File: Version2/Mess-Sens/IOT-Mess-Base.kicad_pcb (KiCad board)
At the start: 2 copper layers, 24.5 x 32.5 mm, 45 parts, among them IC1 SHT40I-AD1F-R2, J1 Conn_01x02_Pin, J2 TP_4056, J4 Conn_01x12_Pin, Q1 NM8205 PFETs, Q5 AO3401A, SW4 SW_Push, SW5 SW_Push, U1 TPL5110, U10 OPT3001DNPR, U11 HDC2010/DSBGA-6, U12 MMC5633NJL/WLP-4, U13 BH1750FVI-TR, U14 T117W, U15 DS1307Z+, U16 ENS210, U17 LIS2MDL, U19 MTS4, U2 INA219AxDCN, U3 TLV493D, U4 INA219AxD, U5 SHT31-DIS, U6 APDS-9960, U7 QMC6309/WLCSP-4, U8 AND_Gate, U9 LTR-303ALS-01

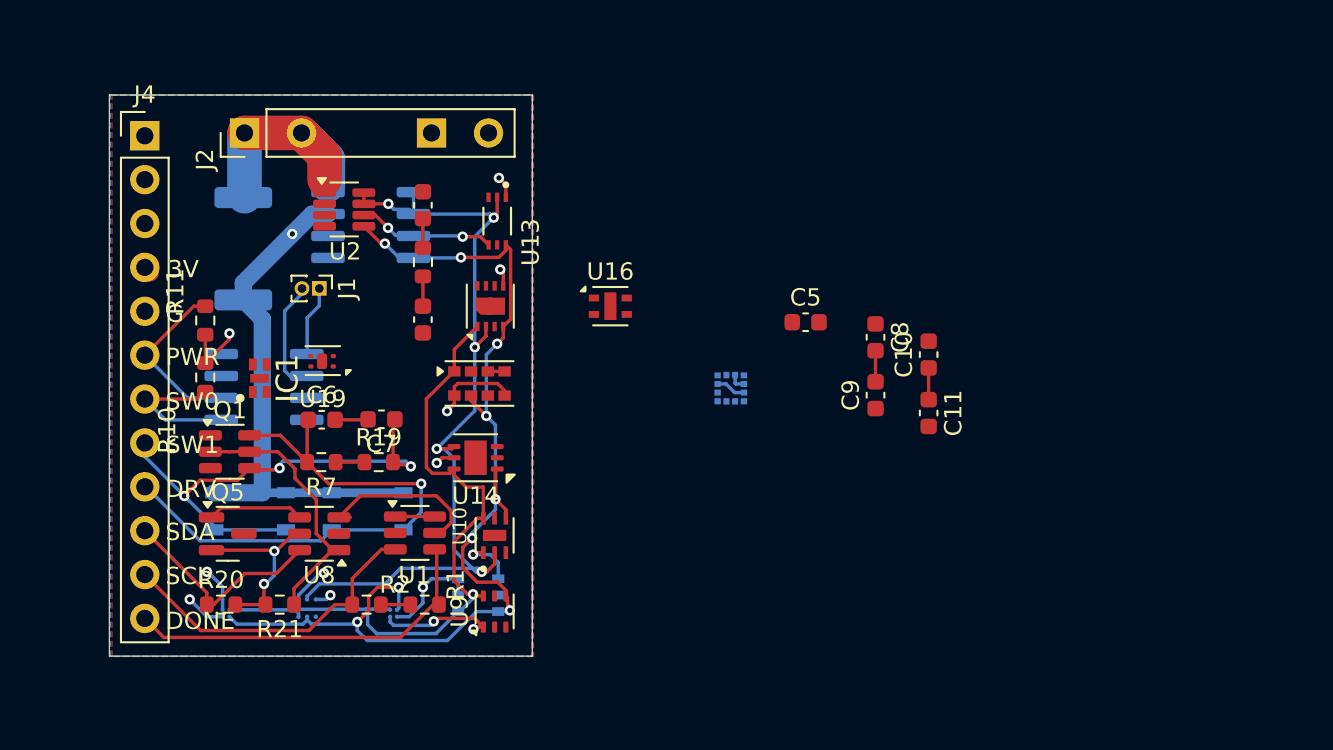
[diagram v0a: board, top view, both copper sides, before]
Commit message: updated.
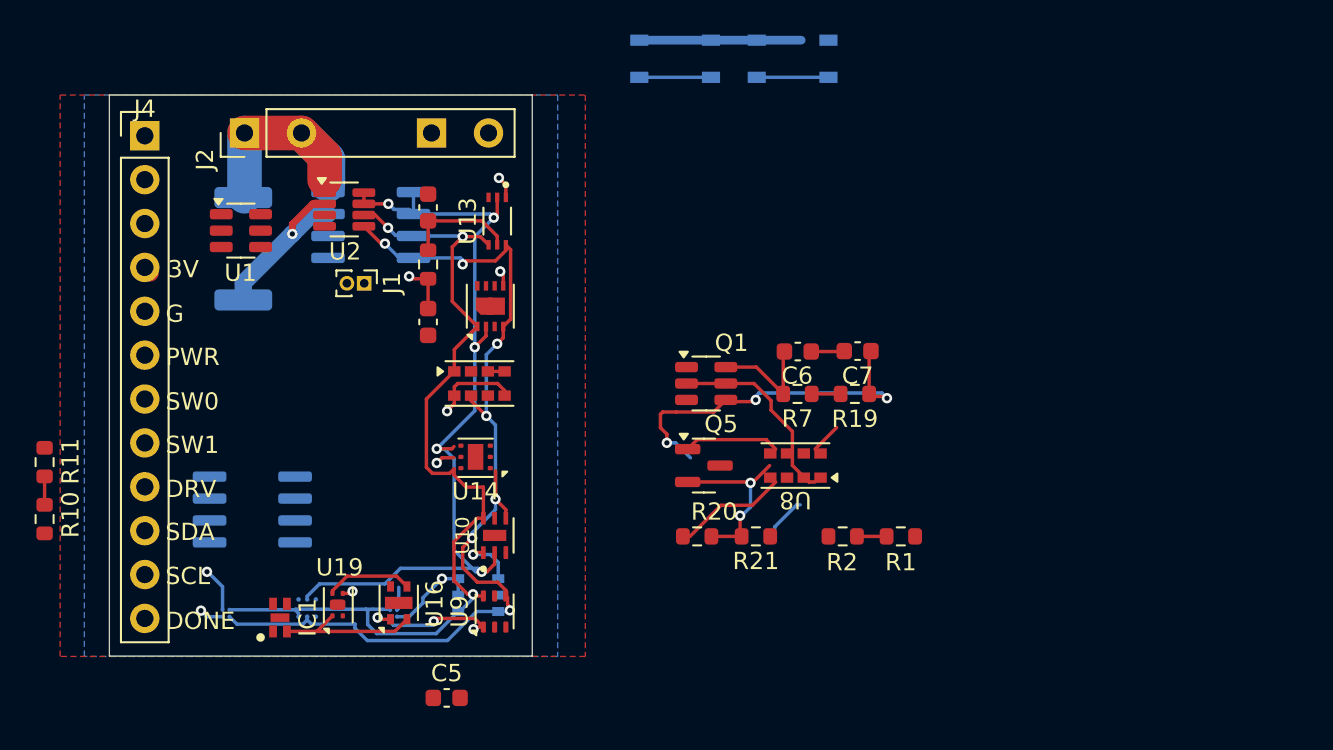
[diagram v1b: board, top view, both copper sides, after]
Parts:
- removed C10, C11: .1u, Capacitor_SMD:C_0603_1608Metric
- removed C8: .22u, Capacitor_SMD:C_0603_1608Metric
- removed C9: 10u, Capacitor_SMD:C_0603_1608Metric
- removed U17: LIS2MDL, Package_LGA:LGA-12_2x2mm_P0.5mm
- U14: footprint Package_DFN_QFN:TDFN-6-1EP_2.5x2.5mm_P0.65mm_EP1.3x2mm -> IOT-Mess-Footprints:DFN-6L
- U8: footprint Package_TO_SOT_SMD:SOT-23-6 -> Sensor:Avago_APDS-9960
- moved SW4 35.9 mm to (118.3, 60.5)
- moved SW5 35.9 mm to (111.5, 60.5)
- moved C5 30.1 mm to (98.3, 97.5)
- moved C7 27.8 mm to (122.1, 77.4)
- moved Q1 27.8 mm to (113.3, 79.3)
- moved Q5 27.8 mm to (113.2, 84.1)
- moved R19 27.8 mm to (121.9, 79.9)
- moved R2 27.8 mm to (121.2, 88.1)
- moved R20 27.8 mm to (112.8, 88.2)
- moved R21 27.8 mm to (116.2, 88.2)
- moved R7 27.8 mm to (118.6, 79.9)
- moved C6 27.8 mm to (118.6, 77.5)
- moved R1 27.8 mm to (124.6, 88.2)
- moved U8 27.8 mm to (118.5, 84.1)
- moved U16 21.1 mm to (95.5, 92.0), turned to 90 degrees
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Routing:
- net LSW0: track 33.4 -> 10.8 mm, vias 1 -> 0
- net DONE: track 21.6 -> 0.18 mm
- net R_DELAY: track 18.7 -> 0.00 mm
- net Vb: track 45.8 -> 30.2 mm
- net Net-(U1-DRV): track 10.3 -> 1.77 mm
- net Net-(J1-Pin_2): track 6.58 -> 0.00 mm
- net EN: track 12.7 -> 6.68 mm
- net SCL_0: track 72.2 -> 67.1 mm, vias 9 -> 7
- net GND: track 17.6 -> 12.6 mm, vias 3 -> 2
- net Net-(U13-DVI): track 1.70 -> 6.57 mm
- net Net-(U8-A): track 15.7 -> 11.3 mm
- net Net-(J1-Pin_1): track 4.10 -> 0.00 mm
- net +3.3V: track 32.7 -> 29.3 mm, vias 10 -> 11
- net LSW1: track 28.6 -> 25.3 mm
- net SDA_0: track 56.6 -> 59.1 mm

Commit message: did some works.
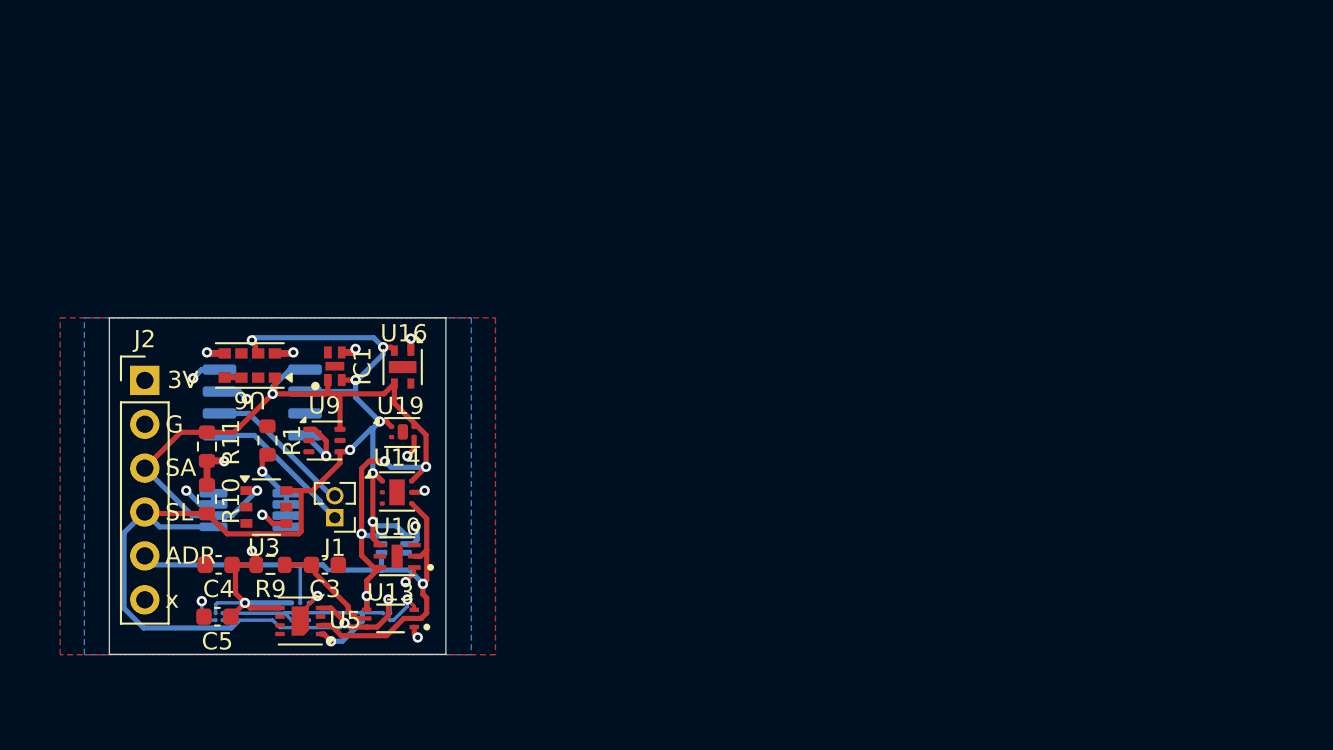
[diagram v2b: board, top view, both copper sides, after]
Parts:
- removed C6, C7: 0.1u, Capacitor_SMD:C_0603_1608Metric
- removed J4: Conn_01x12_Pin, Connector_PinHeader_2.54mm:PinHeader_1x12_P2.54mm_Vertical
- removed Q1: NM8205 PFETs, Package_TO_SOT_SMD:SOT-23-6
- removed Q5: AO3401A, Package_TO_SOT_SMD:SOT-23
- removed R19, R2, R20, R21, R7: R, Resistor_SMD:R_0603_1608Metric
- removed R4: 0.1R, Resistor_SMD:R_2512_6332Metric
- removed SW4, SW5: SW_Push, Button_Switch_SMD:SW_SPST_PTS810
- removed U2: INA219AxDCN, Package_TO_SOT_SMD:SOT-23-8
- removed U8: AND_Gate, Sensor:Avago_APDS-9960
- C3: value 0.1u -> 0.1uF
- C4: value 1u -> 1uF
- J1: footprint Connector_PinHeader_1.00mm:PinHeader_1x02_P1.00mm_Vertical -> Connector_PinHeader_1.27mm:PinHeader_1x02_P1.27mm_Vertical
- J2: value TP_4056 -> Conn_01x06_Pin; footprint IOT-Mess-Footprints:TP_Charger -> Connector_PinHeader_2.54mm:PinHeader_1x06_P2.54mm_Vertical
- R1: value R -> 10K
- U1: value TPL5110 -> TMP102xxDRL; footprint Package_TO_SOT_SMD:SOT-23-6 -> Package_TO_SOT_SMD:SOT-563; moved to B.Cu
- U3: moved to F.Cu
- U4: value INA219AxD -> TMP1075DGK; footprint Package_SO:SOIC-8_3.9x4.9mm_P1.27mm -> Package_SO:VSSOP-8_3x3mm_P0.65mm
- moved R1 37.1 mm to (87.9, 82.6), turned to -90 degrees
- moved U13 23.8 mm to (95.0, 92.9), turned to 180 degrees
- moved C3 21.5 mm to (91.2, 89.8), turned to 0 degrees
- moved U5 21.3 mm to (89.8, 93.0), turned to 180 degrees
- moved U1 20.2 mm to (95.2, 88.6), turned to 180 degrees
- moved R9 19.6 mm to (88.1, 89.8), turned to 0 degrees
- moved C4 18.6 mm to (85.1, 89.8), turned to 180 degrees
- moved U4 17.9 mm to (86.9, 86.6), turned to 0 degrees
- moved J2 15.4 mm to (80.8, 79.1), turned to 0 degrees
- moved IC1 14.9 mm to (91.8, 78.3)
- moved C5 14.1 mm to (85.0, 92.8), turned to 180 degrees
- moved U9 14.0 mm to (91.2, 82.6), turned to 0 degrees
- moved J1 13.7 mm to (91.8, 87.1), turned to 180 degrees
- moved U16 13.7 mm to (95.7, 78.3), turned to -90 degrees
- moved U6 13.3 mm to (86.9, 78.3), turned to 180 degrees
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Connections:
- J2 pad 1: Va -> +3.3V
- J2 pad 2: Va -> GND
- J2 pad 3: unconnected-(J2-Pin_3-Pad3) -> SDA_0
- J2 pad 4: GND -> SCL_0
- R1 pad 1: GND -> unconnected-(R1-Pad1)
- R1 pad 2: DONE -> Net-(U4-A0)
- R10 pad 1: SDA_0 -> SCL_0
- R11 pad 2: SCL_0 -> SDA_0
- U1 pad 1: Vb -> SCL_0
- U1 pad 3: R_DELAY -> unconnected-(U1-ALERT-Pad3)
- U1 pad 4: DONE -> ADDR
- U1 pad 5: Net-(U1-DRV) -> +3.3V
- U1 pad 6: Vb -> SDA_0
- U14 pad 7: (no net) -> GND
- U4 pad 1: ADDR -> SCL_0
- U4 pad 2: ADDR -> SDA_0
- U4 pad 3: SDA_0 -> GND
- U4 pad 4: SCL_0 -> GND
- U4 pad 5: +3.3V -> Net-(U4-A0)
- U4 pad 6: GND -> Net-(U4-A0)
- U4 pad 7: Vb -> Net-(U4-A0)
- U4 pad 8: Va -> +3.3V
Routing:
- net Vb: track 30.2 -> 0.00 mm, vias 3 -> 0
- net LSW1: track 25.3 -> 0.00 mm, vias 3 -> 0
- net ADDR: track 49.6 -> 34.7 mm, vias 5 -> 1
- net SCL_0: track 67.1 -> 81.2 mm, vias 7 -> 9
- net Va: track 13.9 -> 0.00 mm
- net Net-(U8-A): track 11.3 -> 0.00 mm
- net LSW0: track 10.8 -> 0.00 mm
- net Net-(J1-Pin_1): track 0.00 -> 8.71 mm
- net Net-(J1-Pin_2): track 0.00 -> 8.65 mm
- net SDA_0: track 59.1 -> 67.8 mm, vias 3 -> 7
- net EN: track 6.68 -> 0.00 mm
- net Net-(Q5-G): track 5.56 -> 0.00 mm
- net Net-(U4-A0): track 0.00 -> 4.32 mm, vias 0 -> 1
- net Net-(U1-DRV): track 1.77 -> 0.00 mm
- net +3.3V: track 29.3 -> 30.6 mm, vias 11 -> 14
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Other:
- board size 24.5 x 32.5 mm -> 19.5 x 19.5 mm
- board text added: "ADR"
- board text added: "IOT-Mess SENS V2.0 8/18/25"
- board text added: "SA"
- board text added: "SL"
- board text added: "x"
- board text removed: "DONE"
- board text removed: "DRV"
- board text removed: "IOT-Mess SENS V1.0 7/5/25"
- board text removed: "PWR"
- board text removed: "SCL"
- board text removed: "SDA"
- board text removed: "SW0"
- board text removed: "SW1"

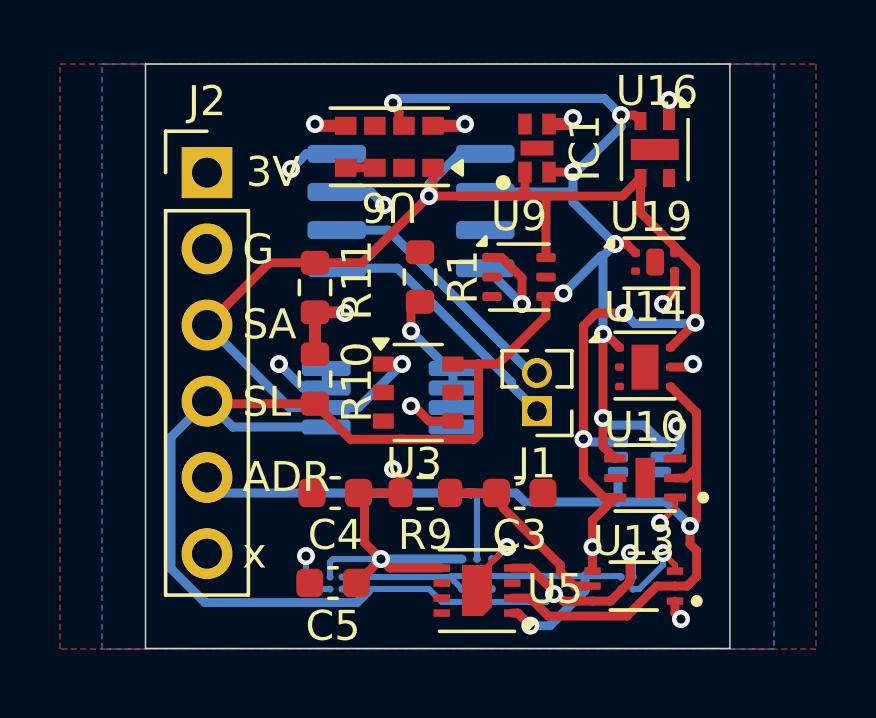
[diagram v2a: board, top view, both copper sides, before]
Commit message: update stuff.
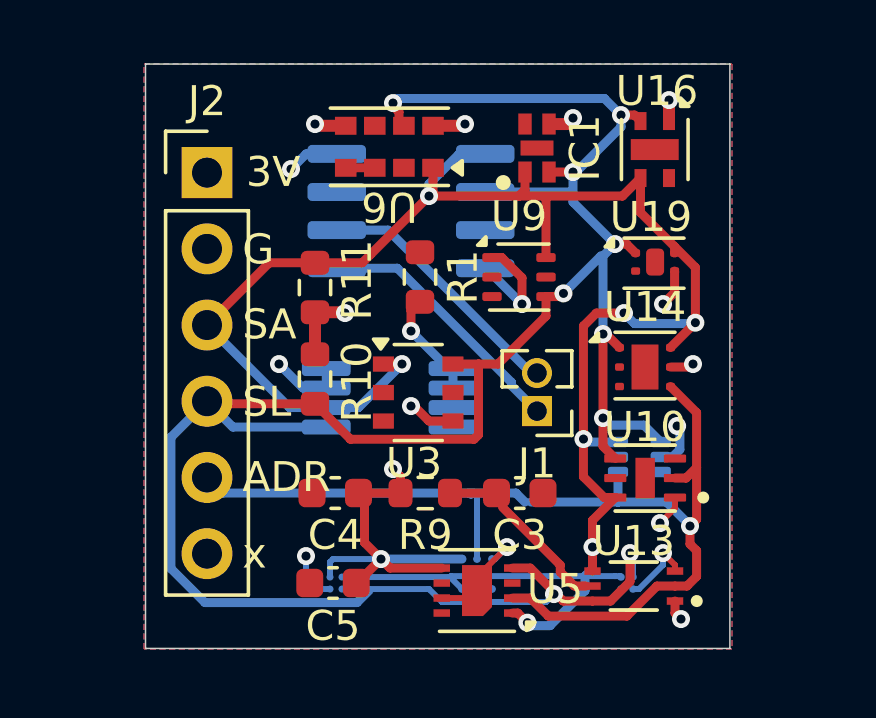
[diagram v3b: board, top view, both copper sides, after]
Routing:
- net +3.3V: track 30.6 -> 28.9 mm, vias 14 -> 13
- net GND: track 12.5 -> 13.8 mm

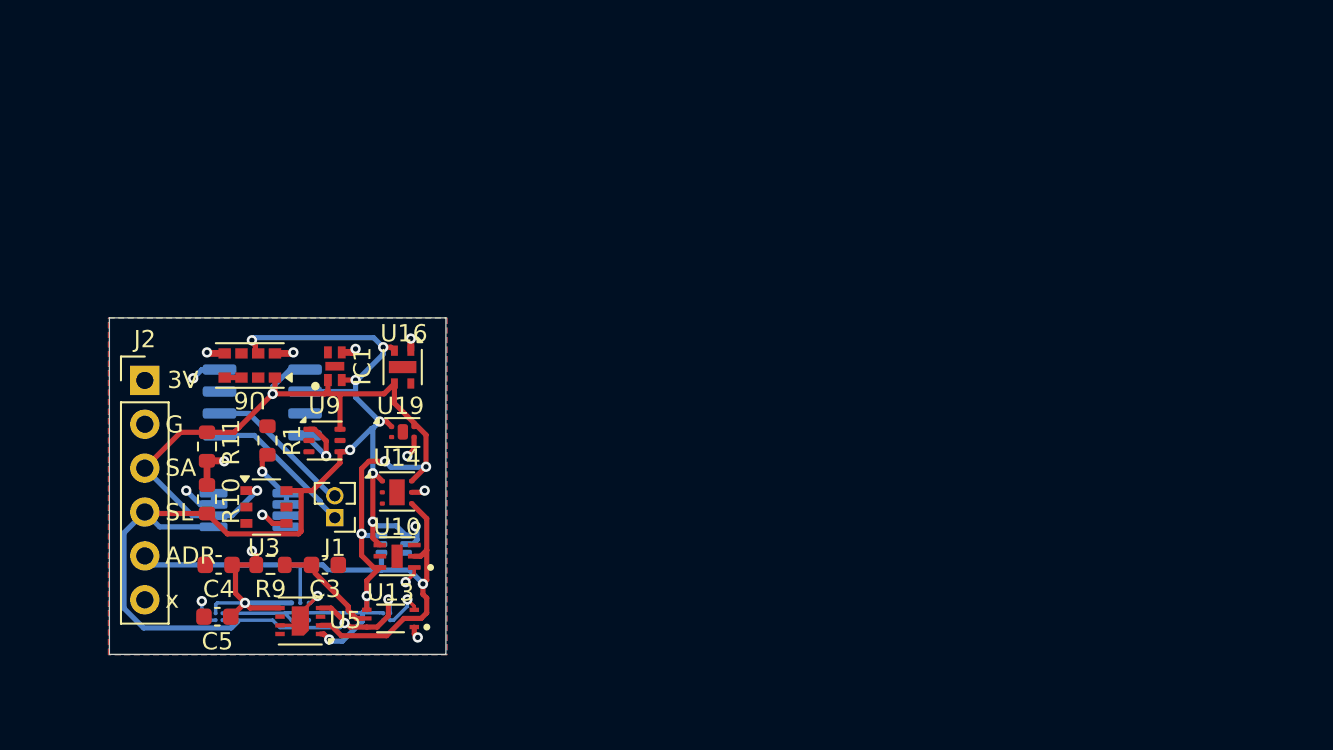
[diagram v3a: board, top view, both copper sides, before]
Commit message: updates.
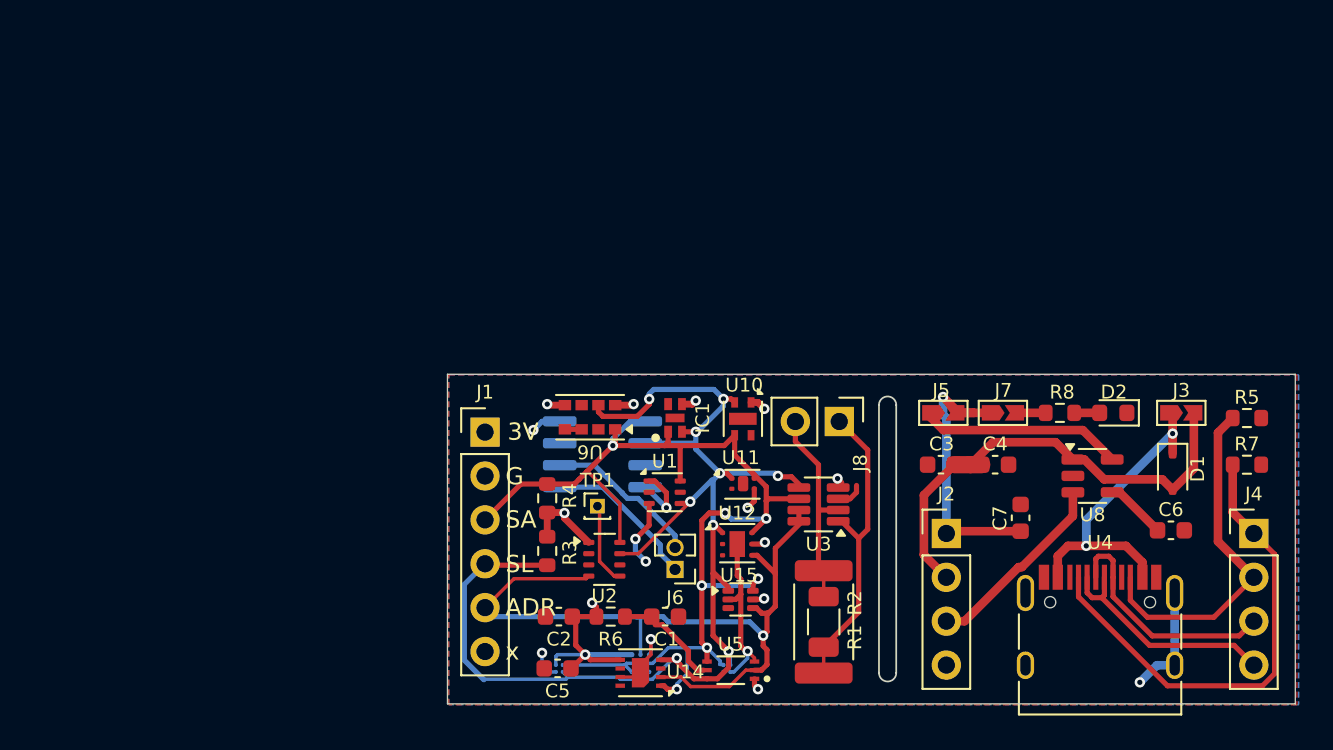
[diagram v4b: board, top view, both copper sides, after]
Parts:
- removed the U10 at (95.4, 89.3)
- added C3: 10u, Capacitor_SMD:C_0603_1608Metric, F.Cu at (126.9, 84.0)
- added C4: 1u, Capacitor_SMD:C_0603_1608Metric, F.Cu at (130.0, 84.0)
- added C6: 22nF, Capacitor_SMD:C_0603_1608Metric, F.Cu at (140.2, 87.8)
- added C7: 1u, Capacitor_SMD:C_0603_1608Metric, F.Cu at (131.5, 87.1)
- added D1: 1N5819WS, Diode_SMD:D_SOD-323, F.Cu at (140.3, 84.4)
- added D2: LED, LED_SMD:LED_0603_1608Metric, F.Cu at (136.9, 81.0)
- added J2: Conn_01x04_Pin, Connector_PinHeader_2.54mm:PinHeader_1x04_P2.54mm_Vertical, F.Cu at (127.2, 88.0)
- added J3: Jumper_2, IOT-Mess-Footprints:Jumpper-triangle, F.Cu at (140.8, 81.0)
- added J4: Conn_01x04_Pin, Connector_PinHeader_2.54mm:PinHeader_1x04_P2.54mm_Vertical, F.Cu at (145.0, 88.0)
- added J5: Jumper_2, IOT-Mess-Footprints:Jumpper-triangle, F.Cu at (127.0, 81.0)
- added J7: Jumper_2, IOT-Mess-Footprints:Jumpper-triangle, F.Cu at (130.5, 81.0)
- added J8: Conn_01x02_Pin, Connector_PinHeader_2.54mm:PinHeader_1x02_P2.54mm_Vertical, F.Cu at (121.0, 81.5)
- added R2: 0.1, Resistor_SMD:R_1206_3216Metric, F.Cu at (120.1, 93.1)
- added R5: 5.1K, Resistor_SMD:R_0603_1608Metric, F.Cu at (144.6, 81.3)
- added R7: 5.1K, Resistor_SMD:R_0603_1608Metric, F.Cu at (144.6, 84.0)
- added R8: R, Resistor_SMD:R_0603_1608Metric, F.Cu at (133.8, 81.0)
- added TP1: TestPoint, Connector_PinHeader_1.00mm:PinHeader_1x01_P1.00mm_Vertical, F.Cu at (107.0, 86.4)
- added U2: LTR-507ALS, IOT-Mess-Footprints:LTR-507ALS, F.Cu at (106.5, 88.5)
- added U8: ME6211C33M5, Package_TO_SOT_SMD:SOT-23-5, F.Cu at (135.7, 84.7)
- R1: value 10K -> 0.1; footprint Resistor_SMD:R_0603_1608Metric -> Resistor_SMD:R_2512_6332Metric
- U1: renamed from U9; value LTR-303ALS-01 -> LTR-303/308
- U11: renamed from U19; value MTS4 -> MTS4 0.1C DFN-4L
- U12: renamed from U14; value T117W -> T117W 0.1C DFN-6L
- U15: renamed from U1; value TMP102xxDRL -> TMP102xxDRL 0.5C SOT-563; moved to F.Cu
- U3: value TLV493D -> INA219AxDCN; footprint Package_SO:TSOP-6_1.65x3.05mm_P0.95mm -> Package_TO_SOT_SMD:SOT-23-8
- U4: value TMP1075DGK -> USB_C_Receptacle_USB2.0_16P; footprint Package_SO:VSSOP-8_3x3mm_P0.65mm -> Connector_USB:USB_C_Receptacle_HRO_TYPE-C-31-M-12; moved to F.Cu
- moved U4 49.8 mm to (136.1, 94.6)
- moved R1 33.9 mm to (120.1, 93.1), turned to 90 degrees
- moved U3 32.0 mm to (119.8, 86.3), turned to 180 degrees
- moved U15 20.3 mm to (115.3, 91.8), turned to 0 degrees
- moved C1 19.9 mm to (110.9, 92.8)
- moved IC1 19.9 mm to (111.5, 81.3)
- moved J1 19.9 mm to (100.5, 82.1)
- moved J6 19.9 mm to (111.5, 90.1)
- moved U10 19.9 mm to (115.4, 81.3)
- moved U13 19.9 mm to (104.7, 95.7)
- moved U14 19.9 mm to (109.5, 96.0)
- moved U16 19.9 mm to (107.3, 83.4)
- moved U7 19.9 mm to (114.5, 95.8)
- moved U9 19.9 mm to (109.5, 95.5)
- moved C2 19.9 mm to (104.8, 92.8)
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- renumbered C3 to C1, C4 to C2, J2 to J1, J1 to J6, R10 to R3, R11 to R4, R9 to R6, U16 to U10, U7 to U13, U5 to U14, U15 to U16, U13 to U5, U12 to U7, U11 to U9
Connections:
- R1 pad 1: unconnected-(R1-Pad1) -> Net-(J8-Pin_1)
- R1 pad 2: Net-(U4-A0) -> Net-(J8-Pin_2)
- U3 pad 1: SDA_0 -> Net-(J8-Pin_1)
- U3 pad 2: GND -> Net-(J8-Pin_2)
- U3 pad 5: unconnected-(U3-GND-Pad5) -> SCL_0
- U3 pad 6: SCL_0 -> SDA_0
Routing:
- net CC1: track 0.00 -> 28.0 mm
- net 5V: track 0.00 -> 27.7 mm
- net CC2: track 0.00 -> 20.3 mm
- net Net-(D1-K): track 0.00 -> 18.6 mm, vias 0 -> 2
- net Net-(J8-Pin_1): track 0.00 -> 17.7 mm
- net +3.3V: track 28.9 -> 45.9 mm, vias 13 -> 14
- net GND: track 13.8 -> 29.8 mm, vias 6 -> 7
- net D+: track 0.00 -> 13.8 mm
- net D-: track 0.00 -> 13.5 mm
- net Net-(J8-Pin_2): track 0.00 -> 12.7 mm
- net Net-(J5-A): track 0.00 -> 11.8 mm
- net CE: track 0.00 -> 11.2 mm
- net ADDR: track 34.7 -> 45.6 mm
- net SCL_0: track 81.0 -> 76.0 mm
- net Net-(U2-VLED): track 0.00 -> 4.78 mm
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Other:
- board size 19.5 x 19.5 mm -> 49.1 x 19.1 mm
